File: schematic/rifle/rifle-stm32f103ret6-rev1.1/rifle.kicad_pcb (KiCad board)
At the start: 2 copper layers, 50.3 x 48 mm, 49 parts, among them K1 Magazine, K2 Fire_mode, K3 IR_LASER, P1 MICROSD-SDIO-CD, P10 RFID-RC522-MODULE, P11 NRF24L01, P12 VibroEng, P13 IR_LED, P14 Power_in, P15 Sound, P16 Indicators, P17 FireFlash, P2 GND, P3 Reset, P4 Reload, P5 Fire, P6 SWD_IO, P7 SWD_CLK, P8 USART2, P9 USART1, Q1 MOSFET_N, Q2 MOS_N, Q4 MOS_N, Q5 MOS_N, U1 3,3 V LDO, U2 5,0 V LDO, U3 STM32F103RE, X1 8MHz

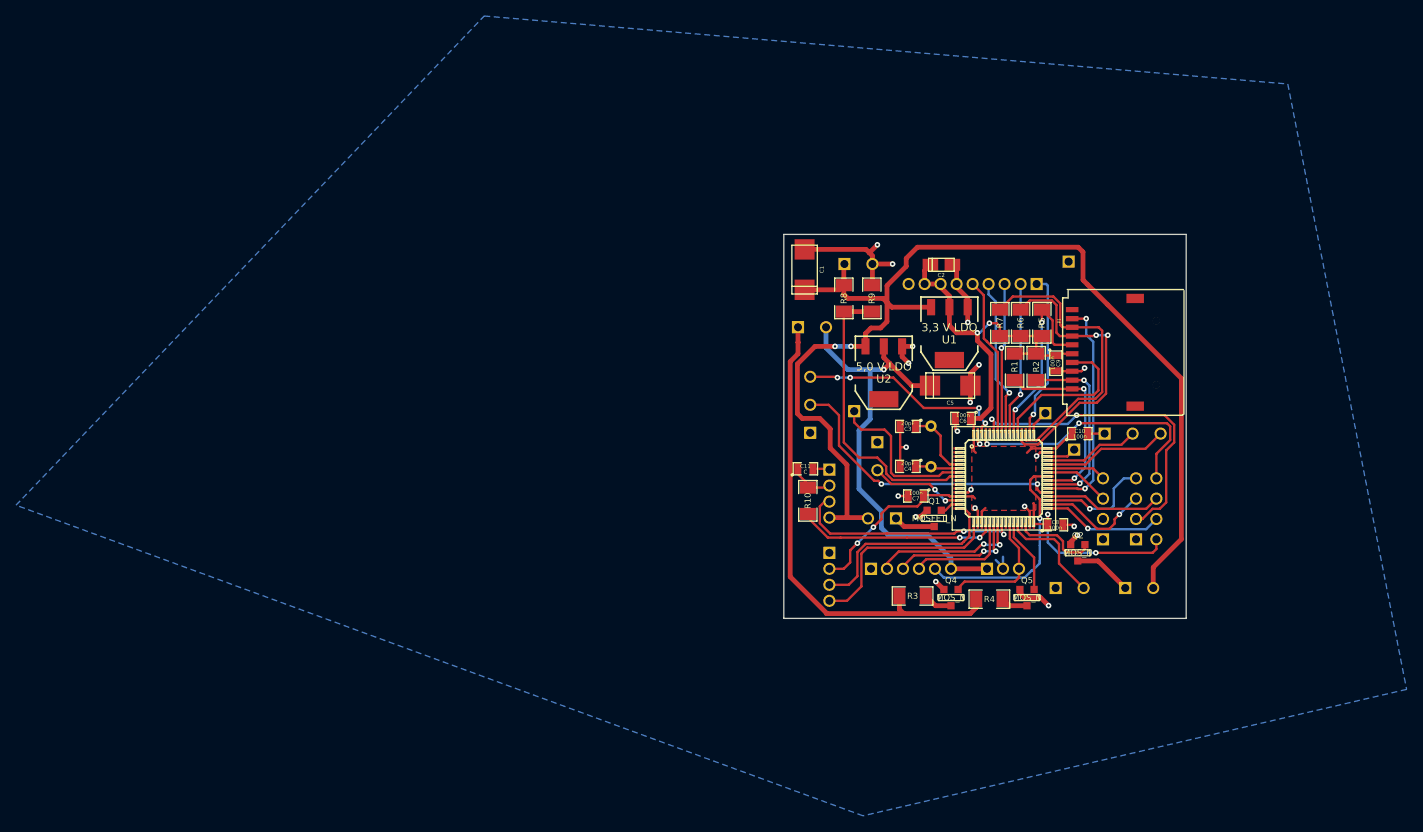
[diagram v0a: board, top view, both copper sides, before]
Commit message: Rifle design seems done
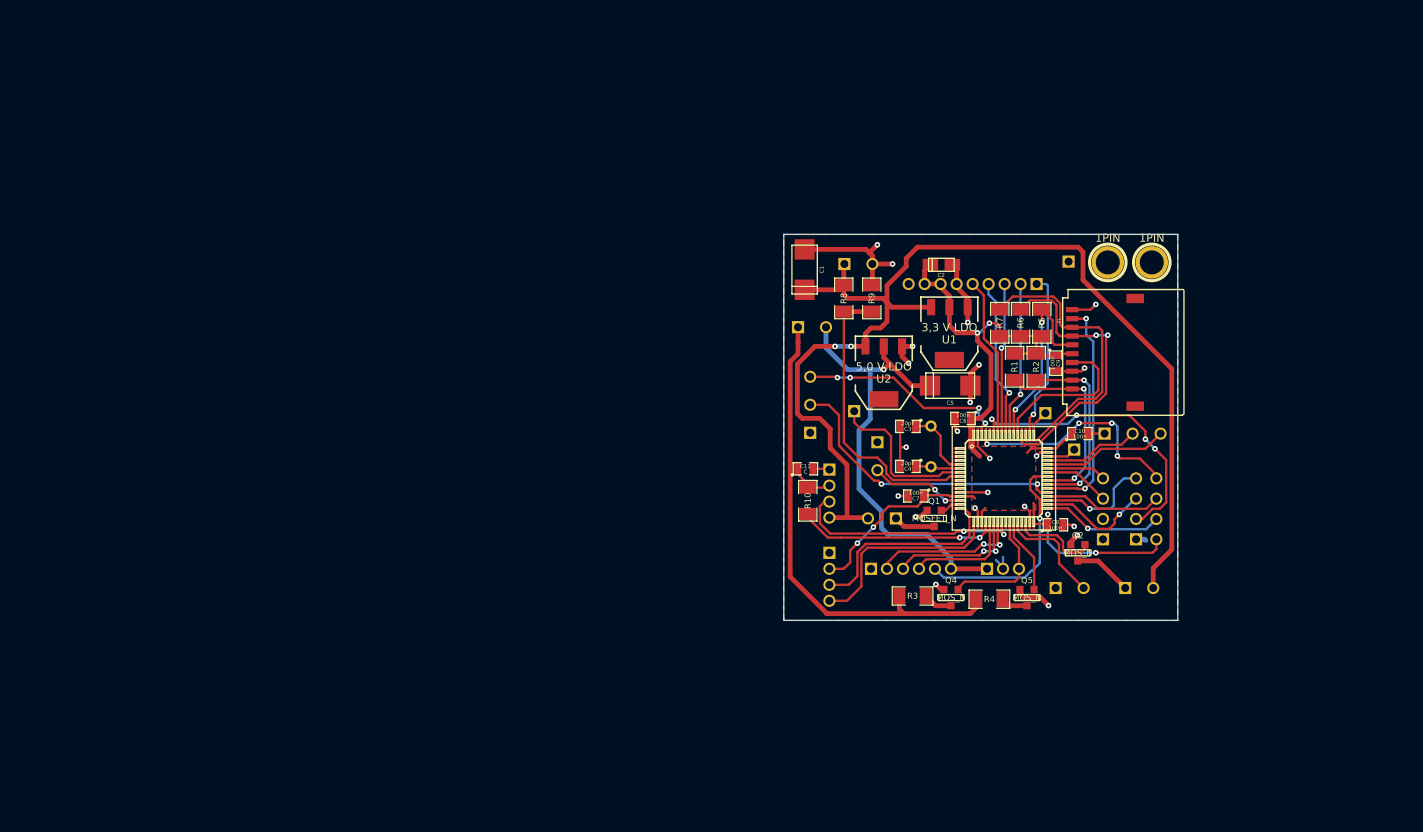
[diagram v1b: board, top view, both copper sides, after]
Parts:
- added 1PIN: P***, 1pin, F.Cu at (109.5, 56.0)
- added 1PIN: P***, 1pin, F.Cu at (104.0, 56.0)
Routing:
- net GND: track 73.6 -> 82.2 mm, vias 21 -> 22
- net +3.3V: track 109.3 -> 114.6 mm
- net N-000009: track 32.8 -> 29.0 mm, vias 2 -> 4
- net N-0000010: track 40.5 -> 37.1 mm, vias 2 -> 4
- net +BATT: track 143.2 -> 142.2 mm
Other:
- board size 50.3 x 48 mm -> 49.2 x 48.2 mm
